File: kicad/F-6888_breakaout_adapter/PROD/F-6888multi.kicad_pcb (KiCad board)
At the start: 2 copper layers, 80.8 x 72.9 mm, 87 parts, among them J1 USB_A, J2 CONN_01X20, J3 MIC, J4 CONN_01X20, J6 Micro_SD_Card_Det, SW1 RESET, SW2 PREV/VOL-, SW3 NEXT/VOL+, SW4 P.P/CALL, SW5 MODE, U1 F-6888

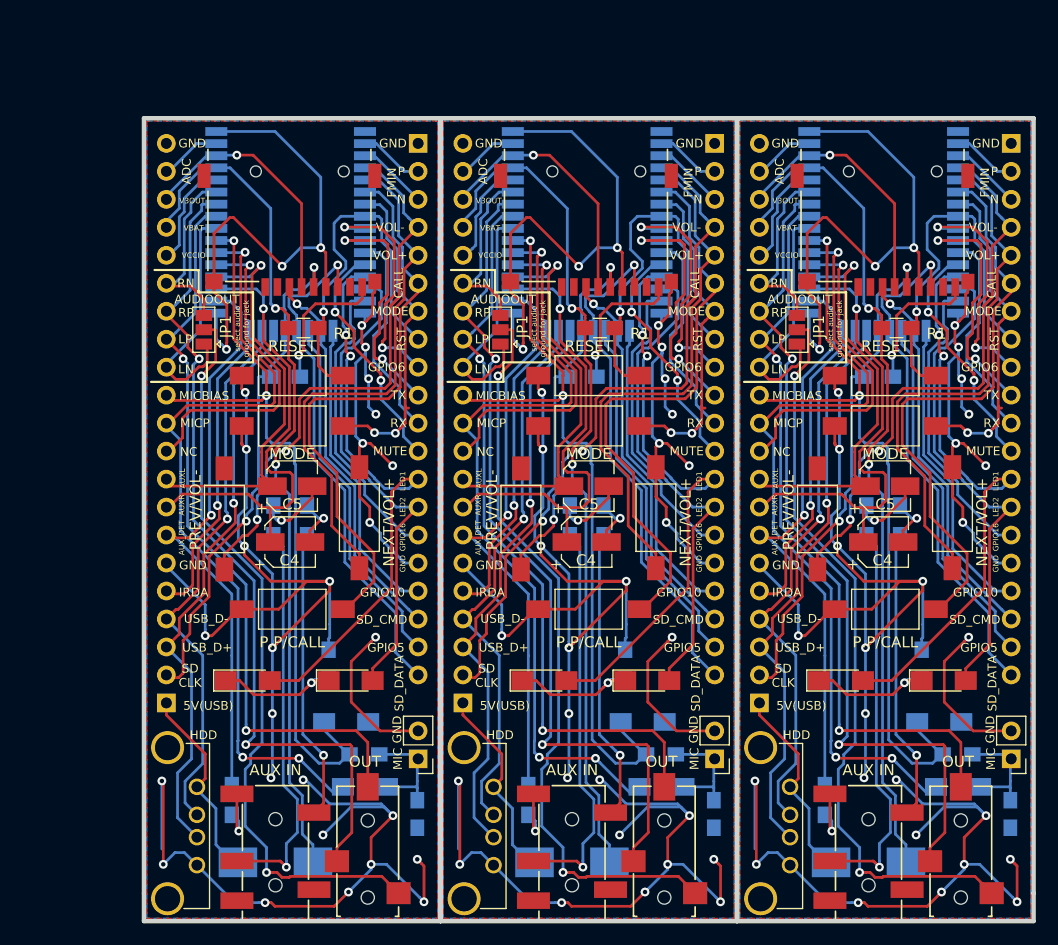
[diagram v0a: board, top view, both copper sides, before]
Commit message: update
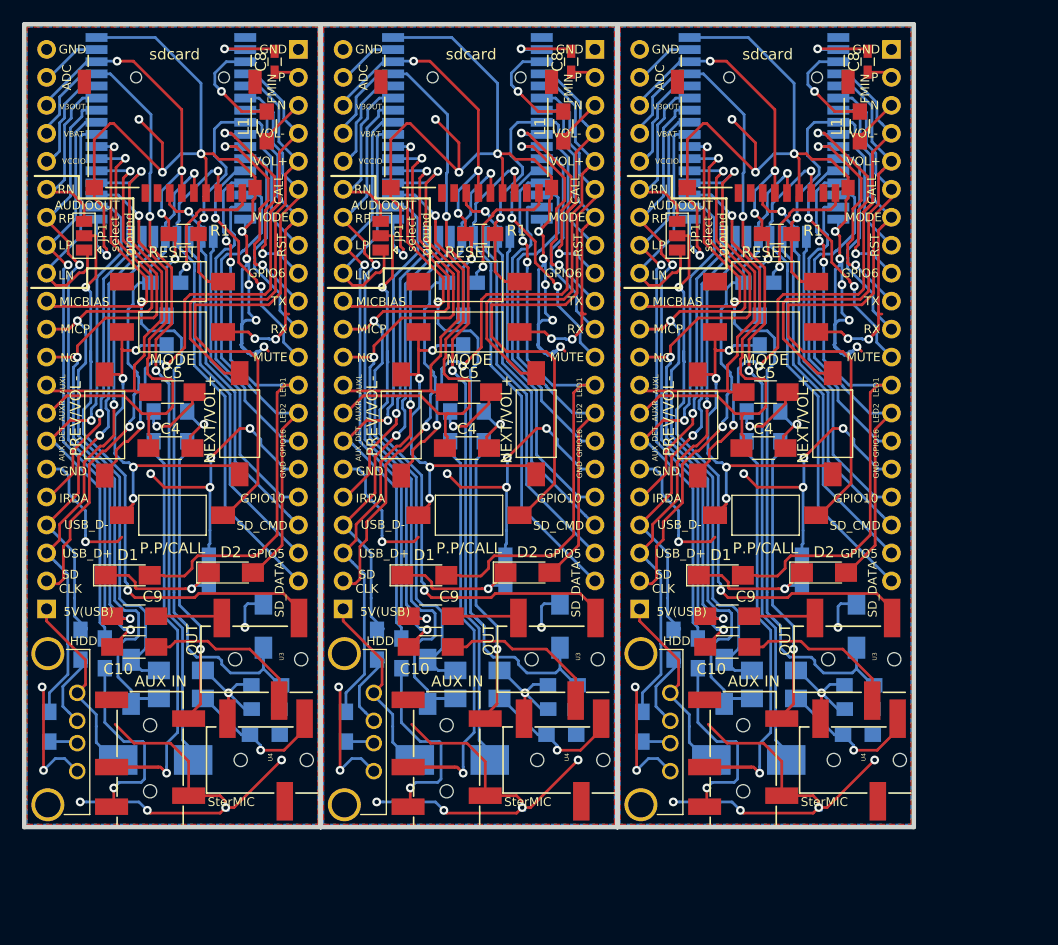
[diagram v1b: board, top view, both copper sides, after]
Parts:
- removed the C1 at (175.3, 116.8)
- removed the C1 at (148.4, 116.8)
- removed the C2 at (177.0, 122.7)
- removed the C2 at (150.1, 122.7)
- removed the C2 at (123.2, 122.7)
- removed the C3 at (181.8, 125.1)
- removed the C3 at (154.9, 125.1)
- removed the C4 at (170.2, 100.5)
- removed the C4 at (143.3, 100.5)
- removed the C4 at (116.4, 100.5)
- removed the C5 at (170.4, 95.4)
- removed the C5 at (143.5, 95.4)
- removed the C5 at (116.6, 95.4)
- removed the D1 at (166.4, 113.0)
- removed the D1 at (139.5, 113.0)
- removed the D2 at (175.7, 113.0)
- removed the D2 at (148.8, 113.0)
- removed the D3 at (168.9, 129.5)
- removed the D3 at (142.0, 129.5)
- removed the J1 at (161.8, 122.7)
- removed the J1 at (134.9, 122.7)
- removed the J1 at (107.9, 122.7)
- removed the J2 at (181.9, 64.3)
- removed the J2 at (154.9, 64.3)
- removed J3 (x3): MIC, Pin_Headers:Pin_Header_Straight_1x02_Pitch2.54mm
- removed the J4 at (159.0, 115.1)
- removed the J4 at (132.1, 115.1)
- removed the J6 at (170.2, 66.8)
- removed the J6 at (143.3, 66.8)
- removed the J6 at (116.3, 66.8)
- removed the JP1 at (162.4, 81.2)
- removed the JP1 at (135.5, 81.2)
- removed PJ-327A1 (x2): CONN_6, jacks:PJ-327A
- removed PJ-327A2 (x3): CONN_6, jacks:3.5mm_stereo_jack_PJ3026
- removed the R1 at (171.4, 81.0)
- removed the R1 at (144.5, 81.0)
- removed the R1 at (117.6, 81.0)
- removed the R2 at (173.7, 111.6)
- removed the R2 at (146.8, 111.6)
- removed the R3 at (177.0, 119.7)
- removed the R3 at (150.1, 119.7)
- removed the R4 at (164.9, 123.9)
- removed the R4 at (138.0, 123.9)
- removed the R5 at (171.8, 98.5)
- removed the R5 at (144.8, 98.5)
- removed the R6 at (168.7, 98.5)
- removed the R6 at (141.8, 98.5)
- removed the R7 at (169.8, 85.4)
- removed the R7 at (142.9, 85.4)
- removed the SW1 at (170.4, 85.3)
- removed the SW1 at (143.5, 85.3)
- removed the SW2 at (164.3, 98.4)
- removed the SW2 at (137.4, 98.4)
- removed the SW3 at (176.5, 98.2)
- removed the SW3 at (149.6, 98.2)
- removed the SW4 at (170.4, 106.6)
- removed the SW4 at (143.5, 106.6)
- removed the SW4 at (116.6, 106.6)
- removed the SW5 at (170.4, 89.9)
- removed the SW5 at (143.5, 89.9)
- removed the U1 at (177.0, 81.3)
- removed the U1 at (150.1, 81.3)
- removed the U1 at (123.2, 81.3)
- added C1: 1uF, Capacitors_SMD:C_1206_HandSoldering, B.Cu at (167.8, 108.1)
- added C1: 1uF, Capacitors_SMD:C_1206_HandSoldering, B.Cu at (140.9, 108.1)
- added C10: 1uF, Capacitors_SMD:C_1206_HandSoldering, F.Cu at (156.1, 110.0)
- added C10: 1uF, Capacitors_SMD:C_1206_HandSoldering, F.Cu at (129.2, 110.0)
- added C10: 1uF, Capacitors_SMD:C_1206_HandSoldering, F.Cu at (102.2, 110.0)
- added C2: 1uF, Capacitors_SMD:C_1206_HandSoldering, B.Cu at (160.3, 112.1)
- added C2: 1uF, Capacitors_SMD:C_1206_HandSoldering, B.Cu at (133.4, 112.1)
- added C2: 1uF, Capacitors_SMD:C_1206_HandSoldering, B.Cu at (106.5, 112.1)
- added C3: 100p, Capacitors_SMD:C_0805_HandSoldering, B.Cu at (168.0, 115.6)
- added C3: 100p, Capacitors_SMD:C_0805_HandSoldering, B.Cu at (141.1, 115.6)
- added C4: 1uF, Capacitors_SMD:C_1206_HandSoldering, F.Cu at (159.4, 91.9)
- added C4: 1uF, Capacitors_SMD:C_1206_HandSoldering, F.Cu at (132.4, 91.9)
- added C4: 1uF, Capacitors_SMD:C_1206_HandSoldering, F.Cu at (105.5, 91.9)
- added C5: 1uF, Capacitors_SMD:C_1206_HandSoldering, F.Cu at (159.6, 86.8)
- added C5: 1uF, Capacitors_SMD:C_1206_HandSoldering, F.Cu at (132.6, 86.8)
- added C5: 1uF, Capacitors_SMD:C_1206_HandSoldering, F.Cu at (105.7, 86.8)
- added C6: 1uF*, Capacitors_SMD:C_1206_HandSoldering, B.Cu at (160.3, 114.7)
- added C6: 1uF*, Capacitors_SMD:C_1206_HandSoldering, B.Cu at (133.4, 114.7)
- added C6: 1uF*, Capacitors_SMD:C_1206_HandSoldering, B.Cu at (106.5, 114.7)
- added C7: 10n(*), Capacitors_SMD:C_1206_HandSoldering, B.Cu at (155.8, 113.2)
- added C7: 10n(*), Capacitors_SMD:C_1206_HandSoldering, B.Cu at (128.9, 113.2)
- added C7: 10n(*), Capacitors_SMD:C_1206_HandSoldering, B.Cu at (102.0, 113.2)
- added C8: 2.2p, Capacitors_SMD:C_0603_HandSoldering, F.Cu at (168.8, 56.8)
- added C8: 2.2p, Capacitors_SMD:C_0603_HandSoldering, F.Cu at (141.9, 56.8)
- added C8: 2.2p, Capacitors_SMD:C_0603_HandSoldering, F.Cu at (115.0, 56.8)
- added C9: 1uF, Capacitors_SMD:C_1206_HandSoldering, F.Cu at (156.1, 107.2)
- added C9: 1uF, Capacitors_SMD:C_1206_HandSoldering, F.Cu at (129.2, 107.2)
- added C9: 1uF, Capacitors_SMD:C_1206_HandSoldering, F.Cu at (102.2, 107.2)
- added D1: LED, LEDs:LED_1206_HandSoldering, F.Cu at (155.5, 103.5)
- added D1: LED, LEDs:LED_1206_HandSoldering, F.Cu at (128.6, 103.5)
- added D2: LED, LEDs:LED_1206_HandSoldering, F.Cu at (164.9, 103.2)
- added D2: LED, LEDs:LED_1206_HandSoldering, F.Cu at (137.9, 103.2)
- added D3: D, Diodes_SMD.pretty:MELF_Handsoldering, B.Cu at (158.0, 120.2)
- added D3: D, Diodes_SMD.pretty:MELF_Handsoldering, B.Cu at (131.1, 120.2)
- added J1: USB_A, modules:USB_A, F.Cu at (150.9, 114.1)
- added J1: USB_A, modules:USB_A, F.Cu at (124.0, 114.1)
- added J1: USB_A, modules:USB_A, F.Cu at (97.1, 114.1)
- added J2: CONN_01X20, Pin_Headers:Pin_Header_Straight_1x20_Pitch2.54mm, B.Cu at (171.0, 55.7)
- added J2: CONN_01X20, Pin_Headers:Pin_Header_Straight_1x20_Pitch2.54mm, B.Cu at (144.1, 55.7)
- added J4: CONN_01X20, Pin_Headers:Pin_Header_Straight_1x21_Pitch2.54mm, B.Cu at (148.1, 106.5)
- added J4: CONN_01X20, Pin_Headers:Pin_Header_Straight_1x21_Pitch2.54mm, B.Cu at (121.2, 106.5)
- added J6: Micro_SD_Card_Det, modules:Conn_uSDcard, F.Cu at (159.3, 58.3)
- added J6: Micro_SD_Card_Det, modules:Conn_uSDcard, F.Cu at (132.4, 58.3)
- added J6: Micro_SD_Card_Det, modules:Conn_uSDcard, F.Cu at (105.5, 58.3)
- added JP1: Jumper_NC_Dual, Jumper:SolderJumper-3_P1.3mm_Open_Pad1.0x1.5mm, F.Cu at (151.5, 72.6)
- added JP1: Jumper_NC_Dual, Jumper:SolderJumper-3_P1.3mm_Open_Pad1.0x1.5mm, F.Cu at (124.6, 72.6)
- added L1: 100nH*, Resistors_SMD.pretty:R_0805_HandSoldering, F.Cu at (168.1, 62.7)
- added L1: 100nH*, Resistors_SMD.pretty:R_0805_HandSoldering, F.Cu at (141.2, 62.7)
- added L1: 100nH*, Resistors_SMD.pretty:R_0805_HandSoldering, F.Cu at (114.3, 62.7)
- added R1: 10k, Resistors_SMD:R_0805_HandSoldering, F.Cu at (160.6, 72.5)
- added R1: 10k, Resistors_SMD:R_0805_HandSoldering, F.Cu at (133.7, 72.5)
- added R1: 10k, Resistors_SMD:R_0805_HandSoldering, F.Cu at (106.7, 72.5)
- added R10: 200, Resistors_SMD:R_0805_HandSoldering, B.Cu at (148.4, 117.2)
- added R10: 200, Resistors_SMD:R_0805_HandSoldering, B.Cu at (121.5, 117.2)
- added R10: 200, Resistors_SMD:R_0805_HandSoldering, B.Cu at (94.5, 117.2)
- added R11: 200, Resistors_SMD:R_0805_HandSoldering, B.Cu at (151.2, 109.8)
- added R11: 200, Resistors_SMD:R_0805_HandSoldering, B.Cu at (124.3, 109.8)
- added R11: 200, Resistors_SMD:R_0805_HandSoldering, B.Cu at (97.4, 109.8)
- added R2: 1k, Resistors_SMD:R_0805_HandSoldering, B.Cu at (162.9, 103.0)
- added R2: 1k, Resistors_SMD:R_0805_HandSoldering, B.Cu at (135.9, 103.0)
- added R3: 1k, Resistors_SMD:R_0805_HandSoldering, B.Cu at (168.1, 113.5)
- added R3: 1k, Resistors_SMD:R_0805_HandSoldering, B.Cu at (141.2, 113.5)
- added R4: 1k, Resistors_SMD:R_0805_HandSoldering, B.Cu at (153.4, 110.6)
- added R4: 1k, Resistors_SMD:R_0805_HandSoldering, B.Cu at (126.5, 110.6)
- added R5: 1k, Resistors_SMD:R_0805_HandSoldering, B.Cu at (160.9, 90.0)
- added R5: 1k, Resistors_SMD:R_0805_HandSoldering, B.Cu at (134.0, 90.0)
- added R6: 1k, Resistors_SMD:R_0805_HandSoldering, B.Cu at (157.8, 90.0)
- added R6: 1k, Resistors_SMD:R_0805_HandSoldering, B.Cu at (130.9, 90.0)
- added R7: 3k3, Resistors_SMD:R_0805_HandSoldering, B.Cu at (158.9, 76.9)
- added R7: 3k3, Resistors_SMD:R_0805_HandSoldering, B.Cu at (132.0, 76.9)
- added R8: 1k*, Resistors_SMD:R_0805_HandSoldering, B.Cu at (167.9, 118.0)
- added R8: 1k*, Resistors_SMD:R_0805_HandSoldering, B.Cu at (141.0, 118.0)
- added R8: 1k*, Resistors_SMD:R_0805_HandSoldering, B.Cu at (114.1, 118.0)
- added R9: 10k, Resistors_SMD:R_0805_HandSoldering, B.Cu at (159.0, 81.3)
- added R9: 10k, Resistors_SMD:R_0805_HandSoldering, B.Cu at (132.1, 81.3)
- added R9: 10k, Resistors_SMD:R_0805_HandSoldering, B.Cu at (105.2, 81.3)
- added SW1: RESET, Buttons_Switches_SMD:SW_SPST_FSMSM, F.Cu at (159.6, 76.8)
- added SW1: RESET, Buttons_Switches_SMD:SW_SPST_FSMSM, F.Cu at (132.6, 76.8)
- added SW2: PREV/VOL-, Buttons_Switches_SMD:SW_SPST_FSMSM, F.Cu at (153.4, 89.8)
- added SW2: PREV/VOL-, Buttons_Switches_SMD:SW_SPST_FSMSM, F.Cu at (126.5, 89.8)
- added SW3: NEXT/VOL+, Buttons_Switches_SMD:SW_SPST_FSMSM, F.Cu at (165.7, 89.7)
- added SW3: NEXT/VOL+, Buttons_Switches_SMD:SW_SPST_FSMSM, F.Cu at (138.7, 89.7)
- added SW4: P.P/CALL, Buttons_Switches_SMD:SW_SPST_FSMSM, F.Cu at (159.6, 98.0)
- added SW4: P.P/CALL, Buttons_Switches_SMD:SW_SPST_FSMSM, F.Cu at (132.6, 98.0)
- added SW4: P.P/CALL, Buttons_Switches_SMD:SW_SPST_FSMSM, F.Cu at (105.7, 98.0)
- added SW5: MODE, Buttons_Switches_SMD:SW_SPST_FSMSM, F.Cu at (159.6, 81.4)
- added SW5: MODE, Buttons_Switches_SMD:SW_SPST_FSMSM, F.Cu at (132.6, 81.4)
- added U1: F-6888, modules:F-6888, B.Cu at (166.2, 72.7)
- added U1: F-6888, modules:F-6888, B.Cu at (139.2, 72.7)
- added U1: F-6888, modules:F-6888, B.Cu at (112.3, 72.7)
- added U2: PJ-327A, jacks:PJ-327A, F.Cu at (157.5, 126.1)
- added U2: PJ-327A, jacks:PJ-327A, F.Cu at (130.6, 126.1)
- added U3: PJ-320B, jacks:3.5mm_stereo_jack_PJ320B, F.Cu at (171.2, 111.1)
- added U3: PJ-320B, jacks:3.5mm_stereo_jack_PJ320B, F.Cu at (144.3, 111.1)
- added U3: PJ-320B, jacks:3.5mm_stereo_jack_PJ320B, F.Cu at (117.4, 111.1)
- added U4: PJ-320B, jacks:3.5mm_stereo_jack_PJ320B, F.Cu at (171.8, 120.2)
- added U4: PJ-320B, jacks:3.5mm_stereo_jack_PJ320B, F.Cu at (144.8, 120.2)
- added U4: PJ-320B, jacks:3.5mm_stereo_jack_PJ320B, F.Cu at (117.9, 120.2)
- R3: value 1k2 -> 1k
- U2: renamed from PJ-327A1; value CONN_6 -> PJ-327A
- moved R4 17.6 mm to (99.6, 110.6)
- moved C3 16.8 mm to (114.2, 115.6), turned to 0 degrees
- moved D2 14.6 mm to (111.0, 103.2)
- moved D1 14.5 mm to (101.7, 103.5)
- moved D3 14.3 mm to (104.2, 120.2)
- moved U2 14.2 mm to (103.7, 126.1)
- moved R2 13.8 mm to (109.0, 103.0)
- moved R5 13.8 mm to (107.0, 90.0)
- moved R6 13.8 mm to (104.0, 90.0)
- moved R7 13.8 mm to (105.1, 76.9)
- moved SW2 13.8 mm to (99.6, 89.8)
- moved SW3 13.8 mm to (111.8, 89.7), turned to 90 degrees
- moved J4 13.8 mm to (94.3, 106.5)
- moved JP1 13.8 mm to (97.7, 72.6)
- moved SW1 13.8 mm to (105.7, 76.8)
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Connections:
- C1 pad 1: GND -> /MICBIAS
- C1 pad 2: /MICBIAS -> GND
- C3 pad 1: GND -> Net-(C2-Pad1)
- C3 pad 2: Net-(C2-Pad1) -> GND
- J2 pad 2: /FMINP -> Net-(C8-Pad1)
- J2 pad 3: /FMINN -> Net-(J2-Pad3)
- R4 pad 2: Net-(PJ-327A1-Pad6) -> Net-(R4-Pad2)
- SW2 pad 1: GND -> Net-(R9-Pad1)
- SW3 pad 1: GND -> Net-(R9-Pad1)
- SW5 pad 1: GND -> Net-(R9-Pad1)
- U2 pad 3: (no net) -> GND
- U2 pad 4: (no net) -> Net-(R4-Pad2)
- U2 pad 6: Net-(PJ-327A1-Pad6) -> (no net)
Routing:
- net GND: track 259.5 -> 182.3 mm, vias 29 -> 21
- net /NC: track 30.3 -> 71.2 mm, vias 1 -> 2
- net Net-(R9-Pad1): track 0.00 -> 35.5 mm, vias 0 -> 4
- net /AUDIORP: track 76.4 -> 54.8 mm
- net (no net): track 3640.1 -> 3660.6 mm, vias 148 -> 154
- net Net-(R4-Pad2): track 0.00 -> 18.3 mm, vias 0 -> 1
- net Net-(C10-Pad1): track 0.00 -> 14.8 mm
- net /V3OUT: track 23.8 -> 38.5 mm, vias 1 -> 4
- net Net-(C6-Pad2): track 0.00 -> 13.3 mm, vias 0 -> 1
- net /AUDIOLP: track 67.9 -> 55.0 mm
- net Net-(JP1-Pad2): track 66.7 -> 54.1 mm
- net /USBD-: track 50.3 -> 40.9 mm
- net /NEXT/VOL+: track 48.3 -> 39.5 mm
- net Net-(J1-Pad2): track 0.00 -> 7.02 mm
- net /MICBIAS: track 69.5 -> 75.7 mm
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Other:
- board text added: "SterMIC"
- board text added: "sdcard"
- board text added: "select ground"
- board text removed: "MIC"
- board text removed: "select audio ground for jack"
